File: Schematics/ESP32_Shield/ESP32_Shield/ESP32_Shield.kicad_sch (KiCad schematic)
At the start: 18 parts, among them J1 Conn_01x10, Q3 Si2319CDS, Q4 Si2319CDS, U6 ADS1234IPW, U7 SHT30-DIS

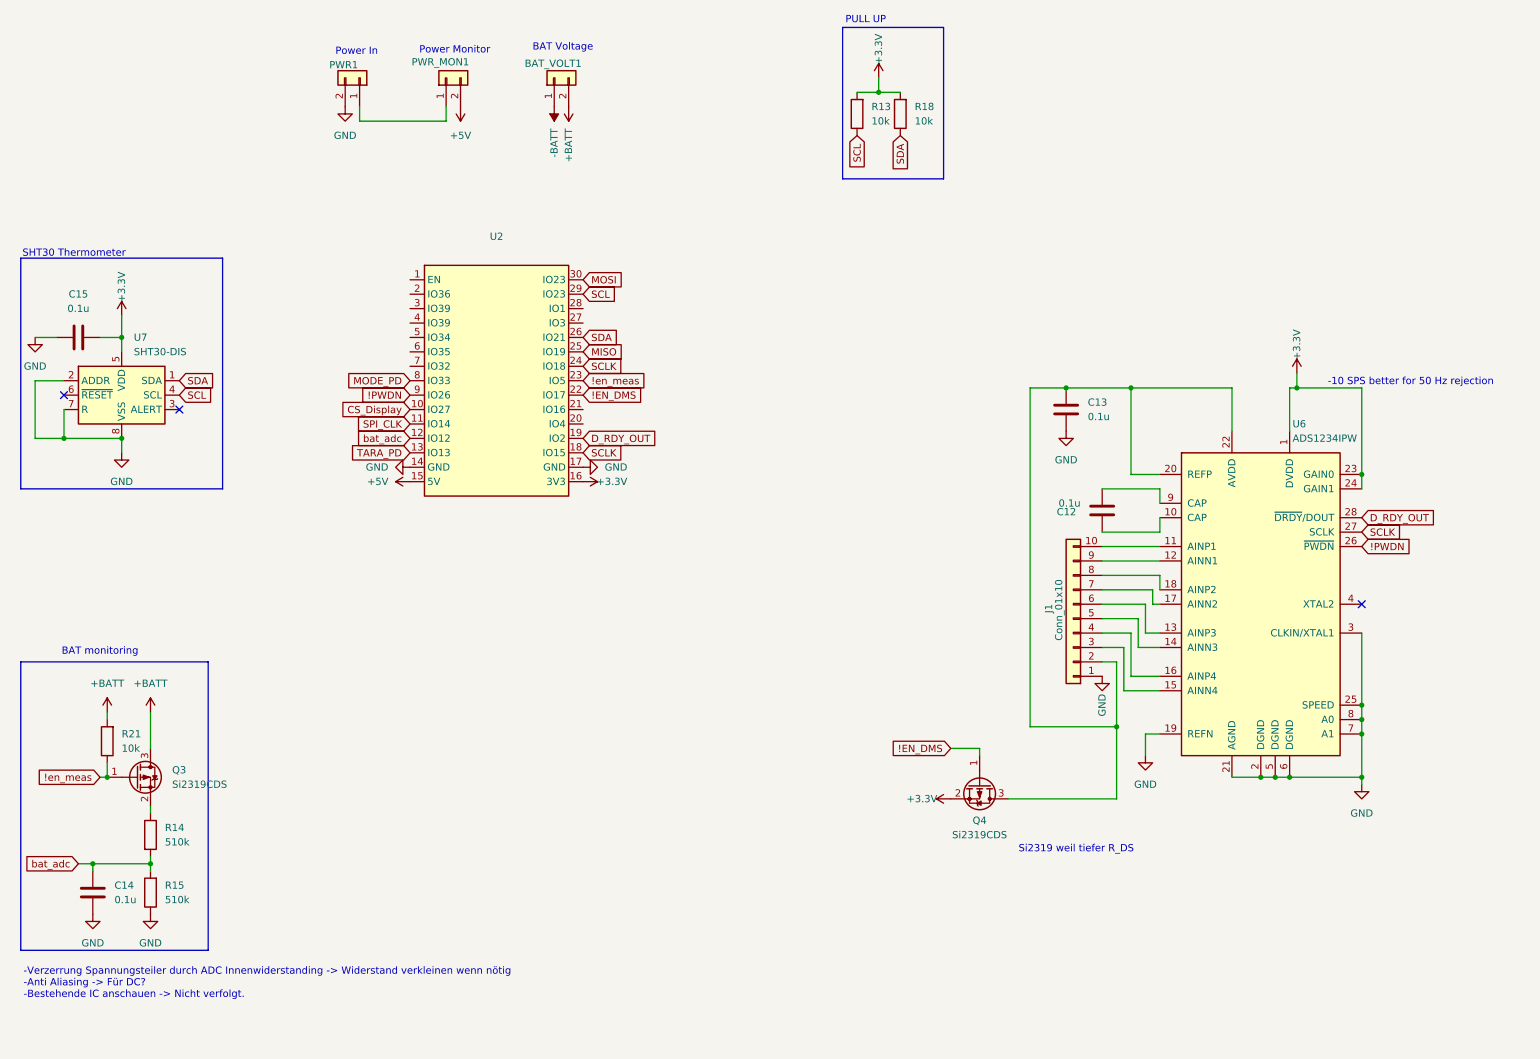
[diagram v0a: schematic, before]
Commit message: kek
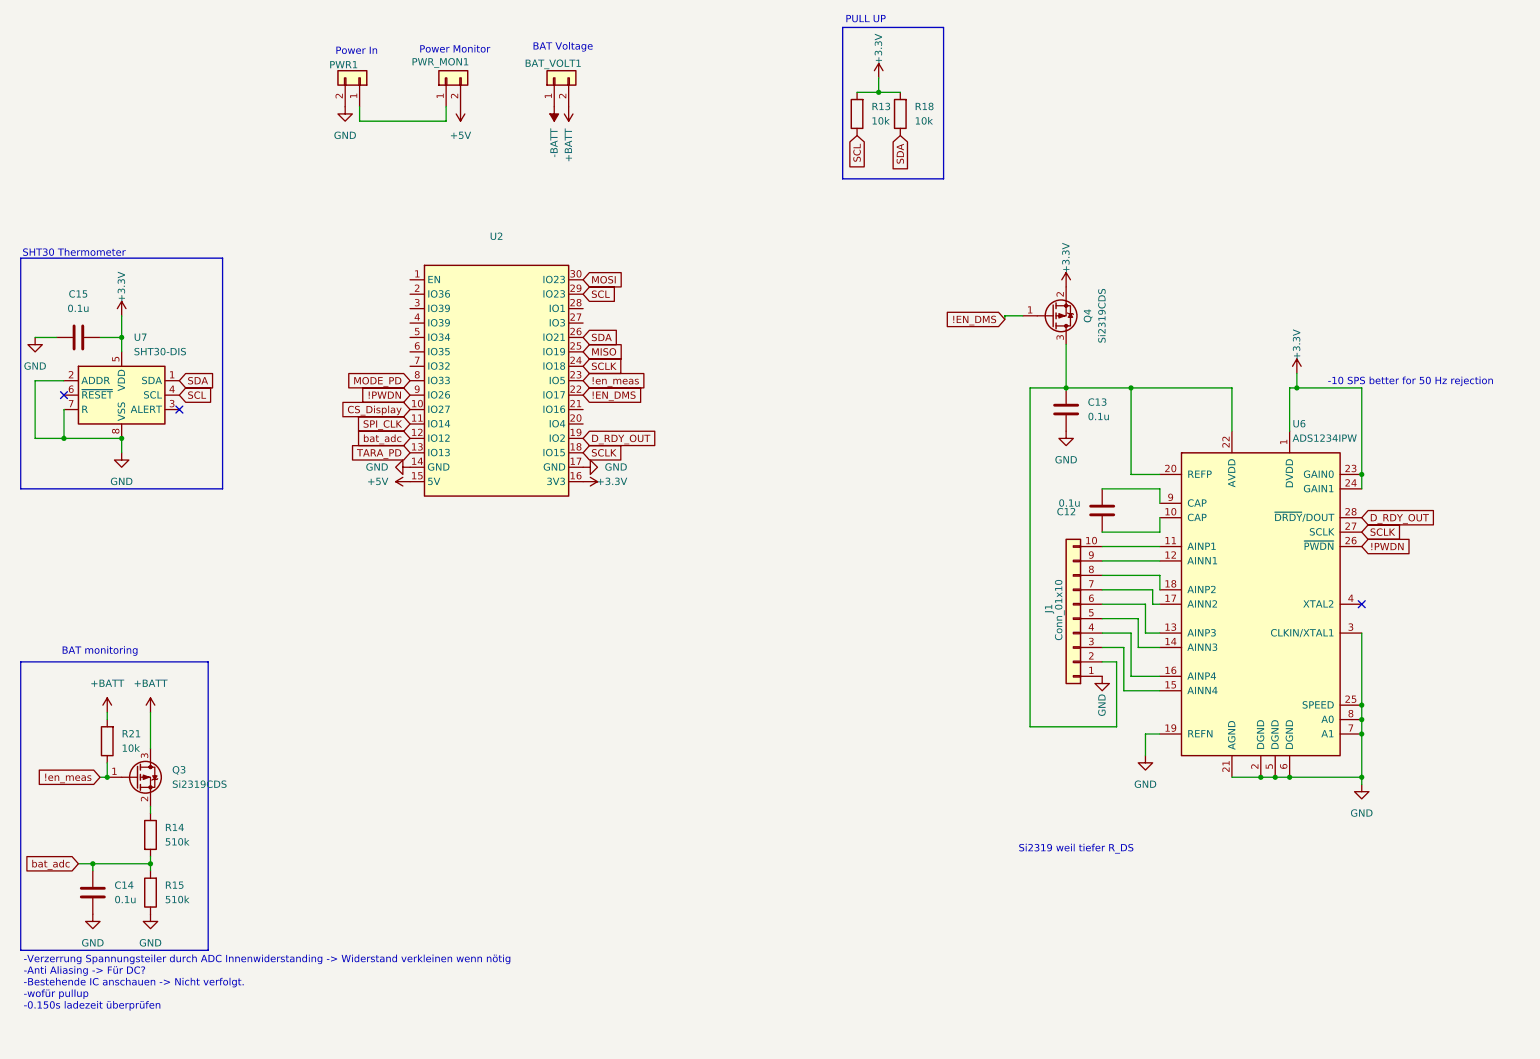
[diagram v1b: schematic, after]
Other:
- note added: "-Verzerrung Spannungsteiler durch ADC Innenwiderstanding -> Widerstand verkleinen wenn nötig -Anti Aliasing -> Für DC? -Bestehende IC anschauen -> Nicht verfolgt. -wofür pullup -0.150s ladezeit überprüfen"
- note removed: "-Verzerrung Spannungsteiler durch ADC Innenwiderstanding -> Widerstand verkleinen wenn nötig -Anti Aliasing -> Für DC? -Bestehende IC anschauen -> Nicht verfolgt."
- moved on the sheet: Q4
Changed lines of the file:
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@@
 		)
 	)
-	(text "-Verzerrung Spannungsteiler durch ADC Innenwiderstanding -> Widerstand verkleinen wenn nötig\n-Anti Aliasing -> Für DC?\n-Bestehende IC anschauen -> Nicht verfolgt.\n\n"
+	(text "-Verzerrung Spannungsteiler durch ADC Innenwiderstanding -> Widerstand verkleinen wenn nötig\n-Anti Aliasing -> Für DC?\n-Bestehende IC anschauen -> Nicht verfolgt.\n-wofür pullup\n-0.150s ladezeit überprüfen\n\n"
 		(exclude_from_sim no)
 		(at 17.018 187.198 0)
@@
 	)
 	(junction
-		(at 209.55 140.97)
-		(diameter 0)
-		(color 0 0 0 0)
-	)
-	(junction
 		(at 234.95 149.86)
 		(diameter 0)
@@
 	(wire
 		(pts
-			(xy 190.5 153.67) (xy 209.55 153.67)
-		)
-		(stroke
-			(width 0)
-			(type default)
-		)
-	)
-	(wire
-		(pts
 			(xy 210.82 134.62) (xy 217.17 134.62)
 		)
@@
 	(wire
 		(pts
+			(xy 200.66 73.66) (xy 200.66 81.28)
+		)
+		(stroke
+			(width 0)
+			(type default)
+		)
+	)
+	(wire
+		(pts
 			(xy 76.2 34.29) (xy 91.44 34.29)
 		)
@@
 	(wire
 		(pts
-			(xy 180.34 144.78) (xy 185.42 144.78)
+			(xy 189.865 69.215) (xy 189.865 68.58)
 		)
 		(stroke
@@
 	(wire
 		(pts
-			(xy 209.55 129.54) (xy 209.55 140.97)
-		)
-		(stroke
-			(width 0)
-			(type default)
-		)
-	)
-	(wire
-		(pts
 			(xy 26.67 165.1) (xy 29.21 165.1)
 		)
@@
 	(wire
 		(pts
-			(xy 209.55 140.97) (xy 209.55 153.67)
+			(xy 209.55 140.97) (xy 209.55 129.54)
 		)
 		(stroke
@@
 	(wire
 		(pts
-			(xy 185.42 144.78) (xy 185.42 146.05)
+			(xy 189.865 68.58) (xy 193.04 68.58)
 		)
 		(stroke
@@
 	(global_label "!EN_DMS"
 		(shape input)
-		(at 180.34 144.78 180)
+		(at 189.865 69.215 180)
 		(fields_autoplaced yes)
 		(effects
@@
 		)
 		(property "Intersheetrefs" "${INTERSHEET_REFS}"
-			(at 169.372 144.78 0)
+			(at 178.897 69.215 0)
 			(effects
 				(font
@@
 	(symbol
 		(lib_id "power:+3.3V")
-		(at 180.34 153.67 90)
-		(mirror x)
+		(at 200.66 63.5 0)
 		(unit 1)
 		(exclude_from_sim no)
@@
 		(dnp no)
 		(property "Reference" "#PWR046"
-			(at 184.15 153.67 0)
+			(at 200.66 67.31 0)
 			(effects
 				(font
@@
 		)
 		(property "Value" "+3.3V"
-			(at 175.26 153.67 90)
+			(at 200.66 58.42 90)
 			(effects
 				(font
@@
 		)
 		(property "Footprint" ""
-			(at 180.34 153.67 0)
+			(at 200.66 63.5 0)
 			(effects
 				(font
@@
 		)
 		(property "Datasheet" ""
-			(at 180.34 153.67 0)
+			(at 200.66 63.5 0)
 			(effects
 				(font
@@
 		)
 		(property "Description" "Power symbol creates a global label with name \"+3.3V\""
-			(at 180.34 153.67 0)
+			(at 200.66 63.5 0)
 			(effects
 				(font
@@
 	(symbol
 		(lib_id "Transistor_FET:Si2319CDS")
-		(at 185.42 151.13 270)
+		(at 198.12 68.58 0)
+		(mirror x)
 		(unit 1)
 		(exclude_from_sim no)
@@
 		(fields_autoplaced yes)
 		(property "Reference" "Q4"
-			(at 185.42 157.48 90)
+			(at 204.47 68.58 90)
 			(effects
 				(font
@@
 		)
 		(property "Value" "Si2319CDS"
-			(at 185.42 160.02 90)
+			(at 207.01 68.58 90)
 			(effects
 				(font
@@
 		)
 		(property "Footprint" "Package_TO_SOT_SMD:SOT-23"
-			(at 183.515 156.21 0)
+			(at 203.2 66.675 0)
 			(effects
 				(font
@@
 		)
 		(property "Datasheet" "http://www.vishay.com/docs/66709/si2319cd.pdf"
-			(at 181.61 156.21 0)
+			(at 203.2 64.77 0)
 			(effects
 				(font
@@
 		)
 		(property "Description" "-4.4A Id, -40V Vds, P-Channel MOSFET, SOT-23"
-			(at 185.42 151.13 0)
-			(effects
-				(font
+			(at 198.12 68.58 0)
+			(effects
+				(font

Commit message: Order ready
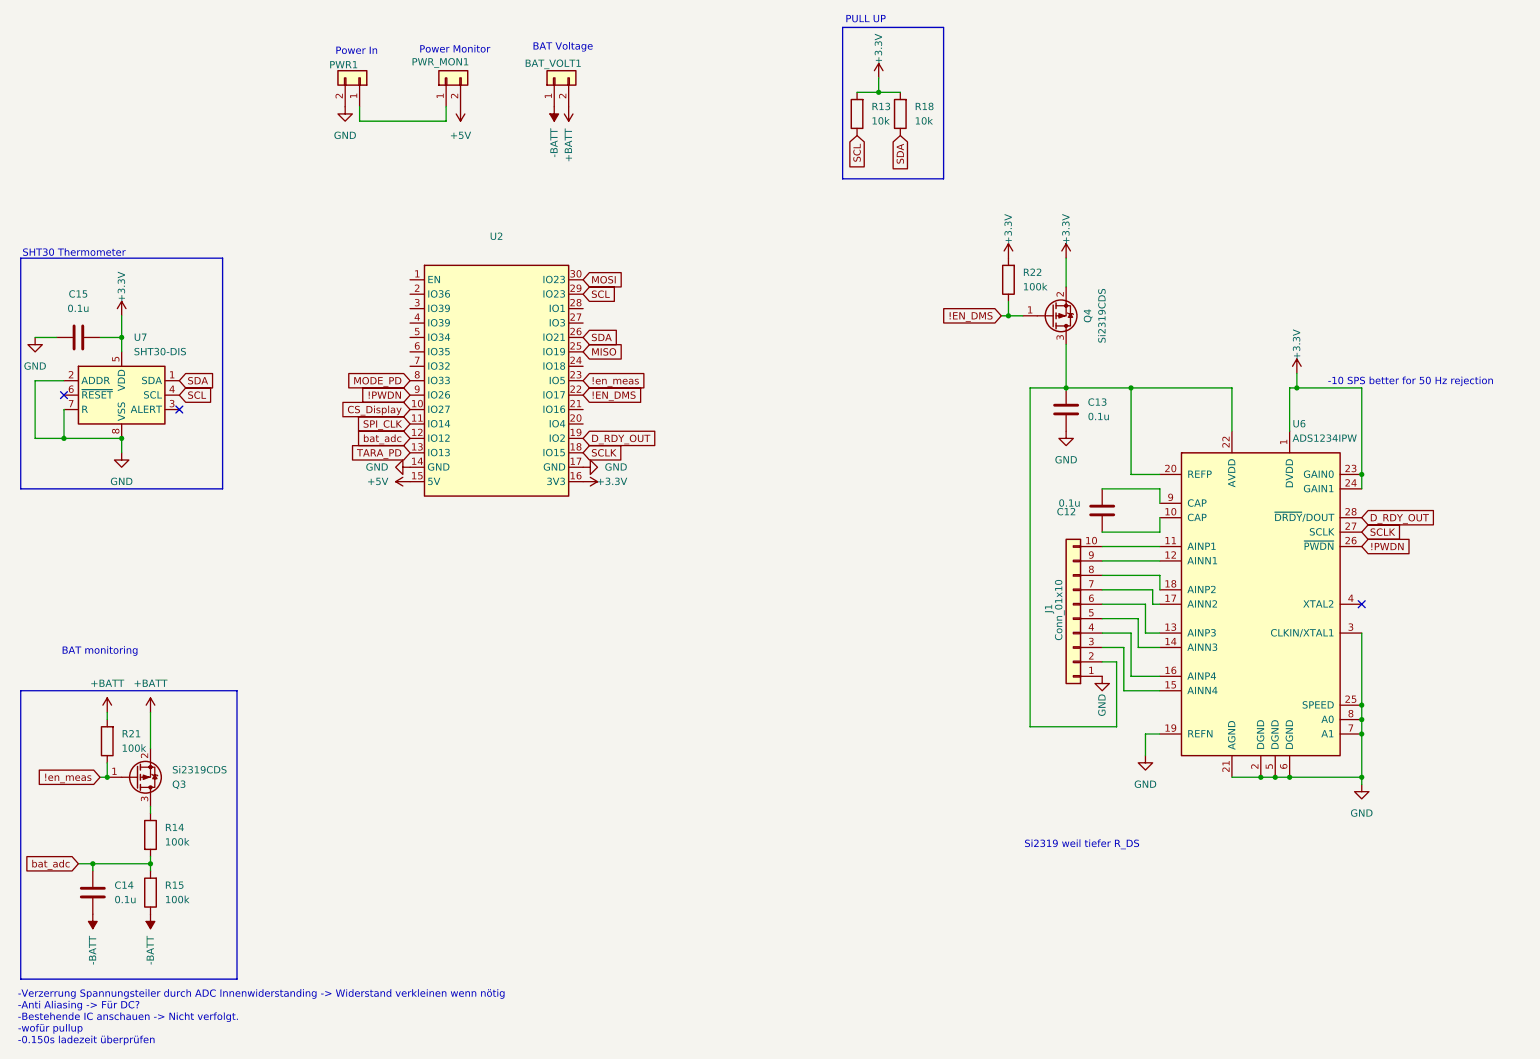
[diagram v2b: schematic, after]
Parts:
- added R22: 100k, Resistor_SMD:R_0603_1608Metric_Pad0.98x0.95mm_HandSolder, symbol Device:R
- R14, R15: value 510k -> 100k
- R21: value 10k -> 100k
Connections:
- net !EN_DMS: now also R22.1
- net +3.3V: now also R22.2
- net +BATT: now also Q3.2 (S); no longer Q3.3 (D)
- net -BATT: now also C14.1, R15.1
- net GND: no longer C14.1, R15.1
- net SCLK: no longer U2.24 (IO18)
- net at R14.1: now also Q3.3 (D); no longer Q3.2 (S)
